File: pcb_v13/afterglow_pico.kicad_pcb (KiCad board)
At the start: 4 copper layers, 70.1 x 88.1 mm, 94 parts, among them J1 USB_B_Micro, J4 Conn_02x17_Odd_Even, J5 Conn_02x17_Odd_Even, SW1 SW_Push, U1 NCP1117-3.3_SOT223, U10 74HC257, U11 74HC257, U2 RP2040, U3 SN74LVC245AN, U4 SN74LVC245AN, U5 W25Q32JVSS, U6 74HC21, U7 7408, U8 74HCT245, U9 74HCT245, Y1 ABLS-12.000MHZ-B4-T

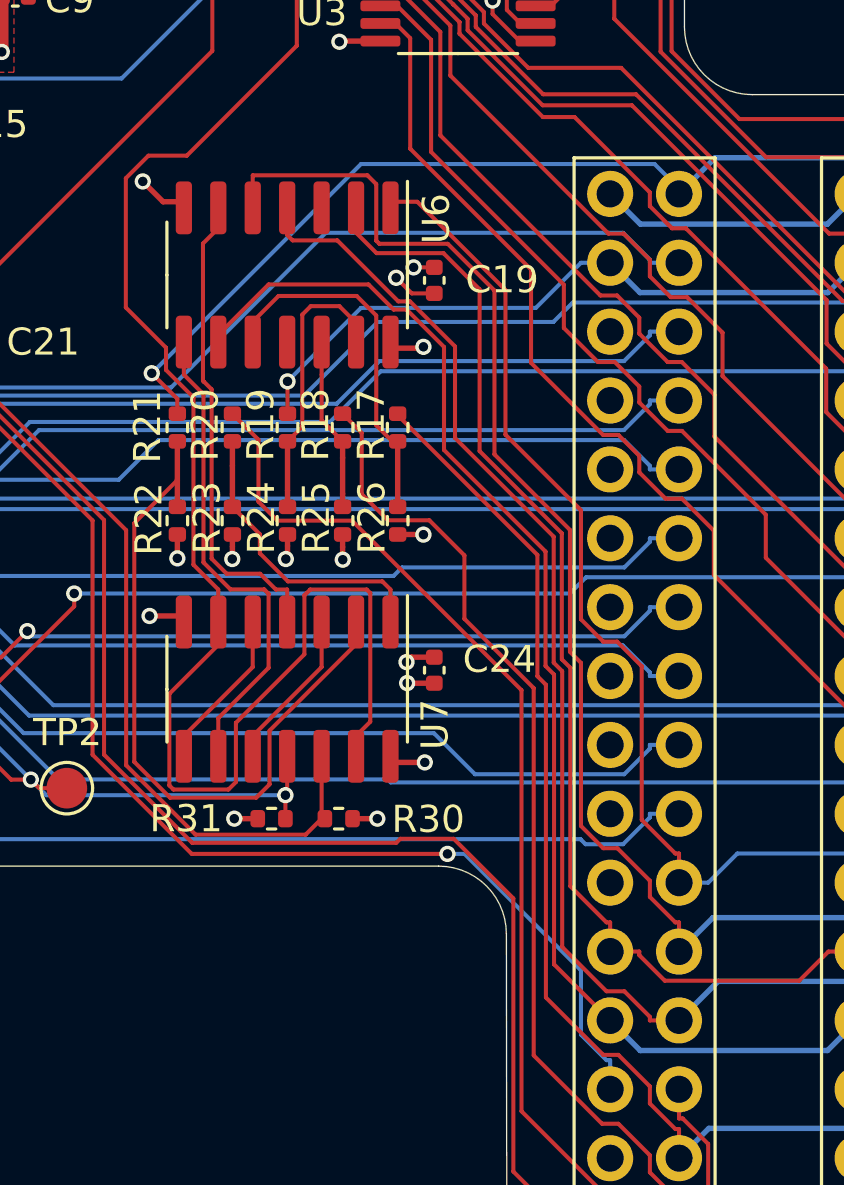
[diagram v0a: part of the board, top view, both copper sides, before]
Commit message: PCB v1.3c
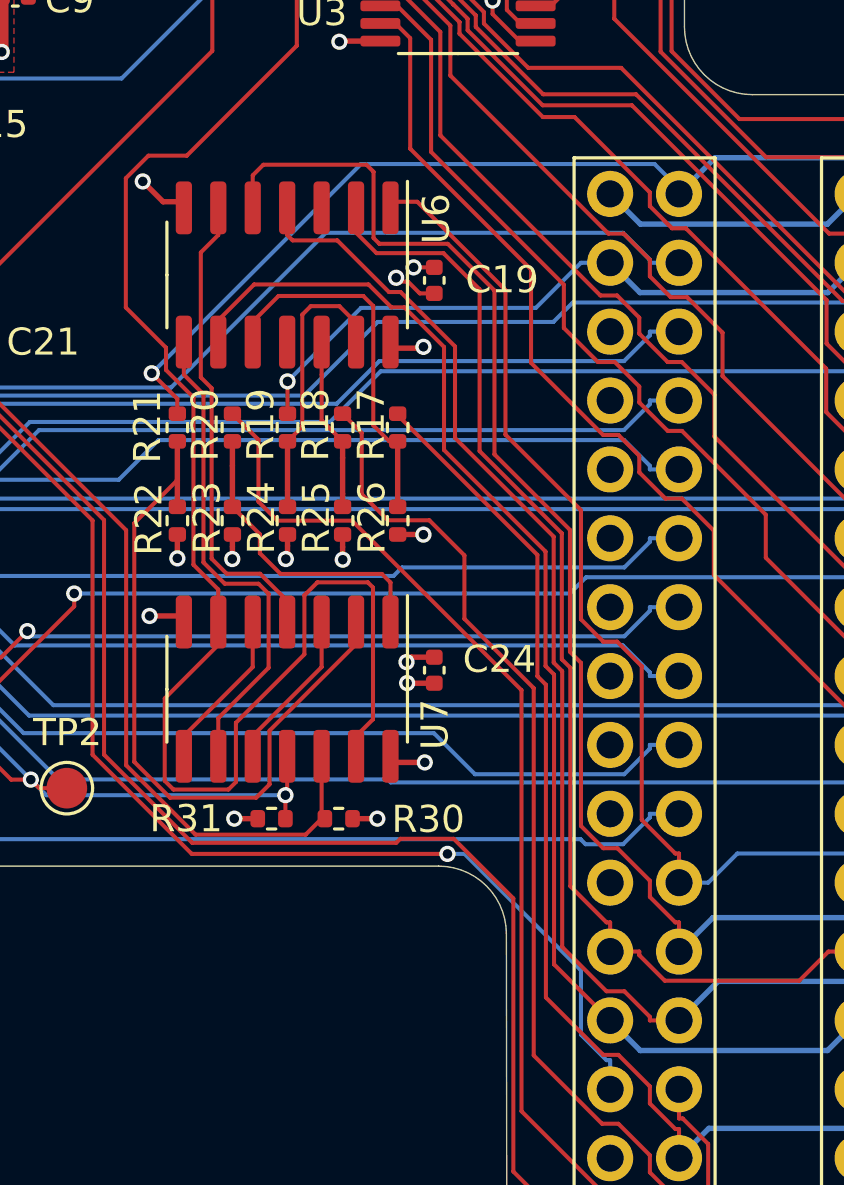
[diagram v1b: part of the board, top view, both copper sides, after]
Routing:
- net Net-(R19-Pad1): track 12.0 -> 11.0 mm
- net /SOL3: track 56.0 -> 56.6 mm
